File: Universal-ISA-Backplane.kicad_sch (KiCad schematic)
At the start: 9 parts

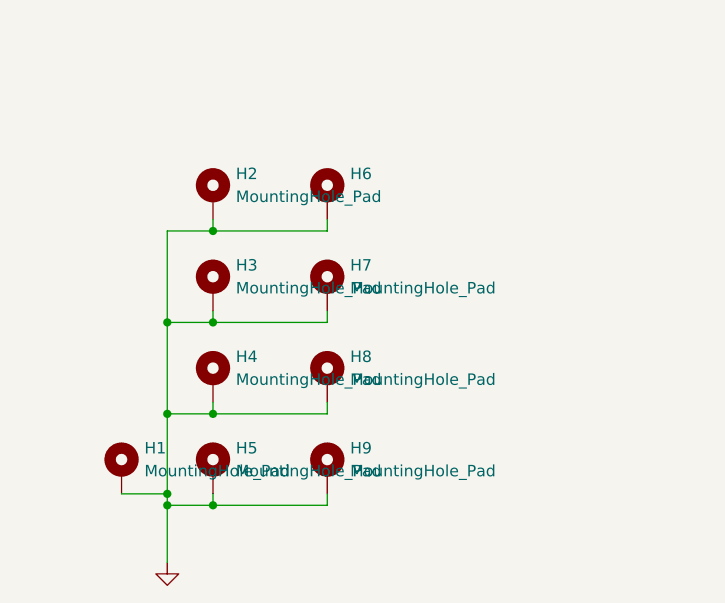
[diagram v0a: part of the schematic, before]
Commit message: Kicad resave fixup
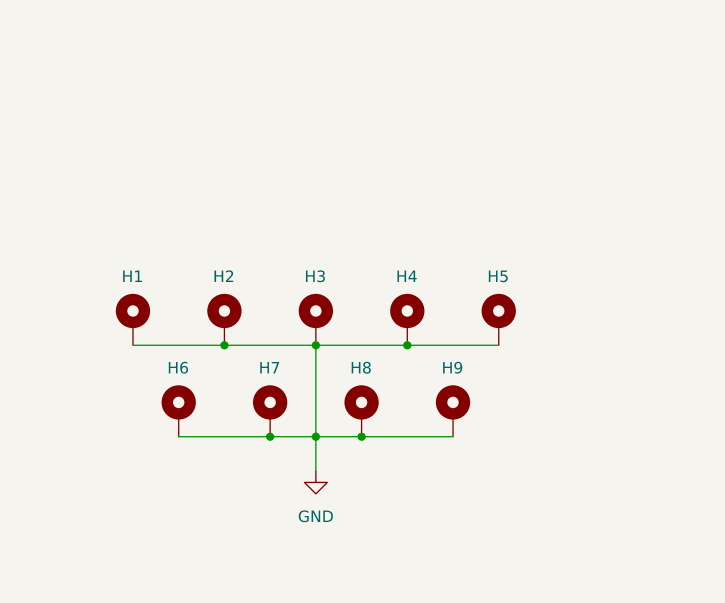
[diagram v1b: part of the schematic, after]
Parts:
- H1, H2, H3, H4, H5, H7, H8, H9: value MountingHole_Pad -> (none)
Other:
- moved on the sheet: H1, H2, H3, H4, H5, H6, H7, H8, H9

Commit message: Just another resave
Not sure why eeschema changed the values and footprints of H1 - H9
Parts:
- H1, H2, H3, H4, H5, H6, H7, H8, H9: value (none) -> MountingHole_Pad; footprint (none) -> MountingHole:MountingHole_4mm_Pad_TopBottom
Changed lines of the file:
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@@
       (effects (font (size 1.27 1.27)) (justify left))
     )
-    (property "Value" "" (id 1) (at 49.53 154.9399 0)
+    (property "Value" "MountingHole_Pad" (id 1) (at 49.53 154.9399 0)
       (effects (font (size 1.27 1.27)) (justify left) hide)
     )
-    (property "Footprint" "" (id 2) (at 46.99 154.94 0)
+    (property "Footprint" "MountingHole:MountingHole_4mm_Pad_TopBottom" (id 2) (at 46.99 154.94 0)
       (effects (font (size 1.27 1.27)) hide)
     )
@@
       (effects (font (size 1.27 1.27)) (justify left))
     )
-    (property "Value" "" (id 1) (at 64.77 165.0999 0)
+    (property "Value" "MountingHole_Pad" (id 1) (at 64.77 165.0999 0)
       (effects (font (size 1.27 1.27)) (justify left) hide)
     )
-    (property "Footprint" "" (id 2) (at 62.23 165.1 0)
+    (property "Footprint" "MountingHole:MountingHole_4mm_Pad_TopBottom" (id 2) (at 62.23 165.1 0)
       (effects (font (size 1.27 1.27)) hide)
     )
@@
       (effects (font (size 1.27 1.27)) (justify left))
     )
-    (property "Value" "" (id 1) (at 29.21 154.9399 0)
+    (property "Value" "MountingHole_Pad" (id 1) (at 29.21 154.9399 0)
       (effects (font (size 1.27 1.27)) (justify left) hide)
     )
-    (property "Footprint" "" (id 2) (at 26.67 154.94 0)
+    (property "Footprint" "MountingHole:MountingHole_4mm_Pad_TopBottom" (id 2) (at 26.67 154.94 0)
       (effects (font (size 1.27 1.27)) hide)
     )
@@
       (effects (font (size 1.27 1.27)) (justify left))
     )
-    (property "Value" "" (id 1) (at 44.45 165.0999 0)
+    (property "Value" "MountingHole_Pad" (id 1) (at 44.45 165.0999 0)
       (effects (font (size 1.27 1.27)) (justify left) hide)
     )
-    (property "Footprint" "" (id 2) (at 41.91 165.1 0)
+    (property "Footprint" "MountingHole:MountingHole_4mm_Pad_TopBottom" (id 2) (at 41.91 165.1 0)
       (effects (font (size 1.27 1.27)) hide)
     )
@@
       (effects (font (size 1.27 1.27)) (justify left))
     )
-    (property "Value" "" (id 1) (at 69.85 154.9399 0)
+    (property "Value" "MountingHole_Pad" (id 1) (at 69.85 154.9399 0)
       (effects (font (size 1.27 1.27)) (justify left) hide)
     )
-    (property "Footprint" "" (id 2) (at 67.31 154.94 0)
+    (property "Footprint" "MountingHole:MountingHole_4mm_Pad_TopBottom" (id 2) (at 67.31 154.94 0)
       (effects (font (size 1.27 1.27)) hide)
     )
@@
       (effects (font (size 1.27 1.27)) (justify left))
     )
-    (property "Value" "" (id 1) (at 59.69 154.9399 0)
+    (property "Value" "MountingHole_Pad" (id 1) (at 59.69 154.9399 0)
       (effects (font (size 1.27 1.27)) (justify left) hide)
     )
-    (property "Footprint" "" (id 2) (at 57.15 154.94 0)
+    (property "Footprint" "MountingHole:MountingHole_4mm_Pad_TopBottom" (id 2) (at 57.15 154.94 0)
       (effects (font (size 1.27 1.27)) hide)
     )
@@
       (effects (font (size 1.27 1.27)) (justify right))
     )
-    (property "Value" "" (id 1) (at 39.37 154.9399 0)
+    (property "Value" "MountingHole_Pad" (id 1) (at 39.37 154.9399 0)
       (effects (font (size 1.27 1.27)) (justify right) hide)
     )
-    (property "Footprint" "" (id 2) (at 36.83 154.94 0)
+    (property "Footprint" "MountingHole:MountingHole_4mm_Pad_TopBottom" (id 2) (at 36.83 154.94 0)
       (effects (font (size 1.27 1.27)) hide)
     )
@@
       (effects (font (size 1.27 1.27)) (justify left))
     )
-    (property "Value" "" (id 1) (at 34.29 165.0999 0)
+    (property "Value" "MountingHole_Pad" (id 1) (at 34.29 165.0999 0)
       (effects (font (size 1.27 1.27)) (justify left) hide)
     )
-    (property "Footprint" "" (id 2) (at 31.75 165.1 0)
+    (property "Footprint" "MountingHole:MountingHole_4mm_Pad_TopBottom" (id 2) (at 31.75 165.1 0)
       (effects (font (size 1.27 1.27)) hide)
     )
@@
       (effects (font (size 1.27 1.27)) (justify left))
     )
-    (property "Value" "" (id 1) (at 54.61 165.0999 0)
+    (property "Value" "MountingHole_Pad" (id 1) (at 54.61 165.0999 0)
       (effects (font (size 1.27 1.27)) (justify left) hide)
     )
-    (property "Footprint" "" (id 2) (at 52.07 165.1 0)
+    (property "Footprint" "MountingHole:MountingHole_4mm_Pad_TopBottom" (id 2) (at 52.07 165.1 0)
       (effects (font (size 1.27 1.27)) hide)
     )
